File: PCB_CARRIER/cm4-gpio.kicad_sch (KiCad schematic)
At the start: 35 parts, among them J2 Micro_SD_Card_Det2, Q1 BSS138, Q3 BSS138, Q4 BC817-40, Q5 BSS138, SW1 SW_DIP_x04, U4 RT9742GGJ5

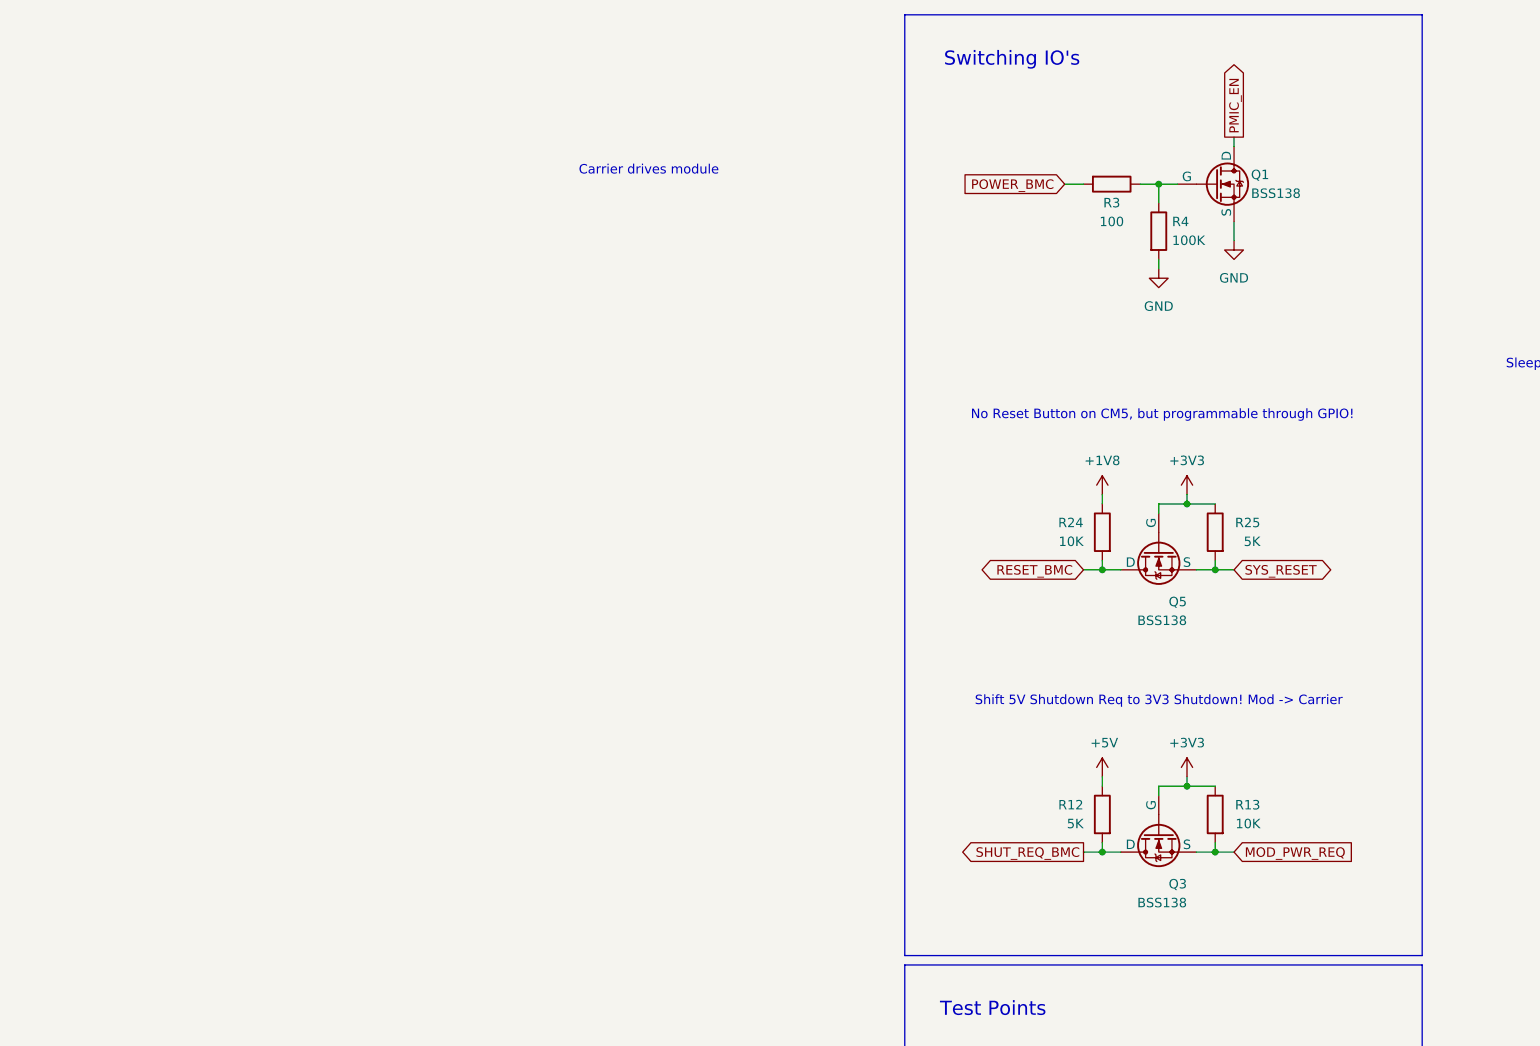
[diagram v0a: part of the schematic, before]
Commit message: fixing the PMIC mosfet
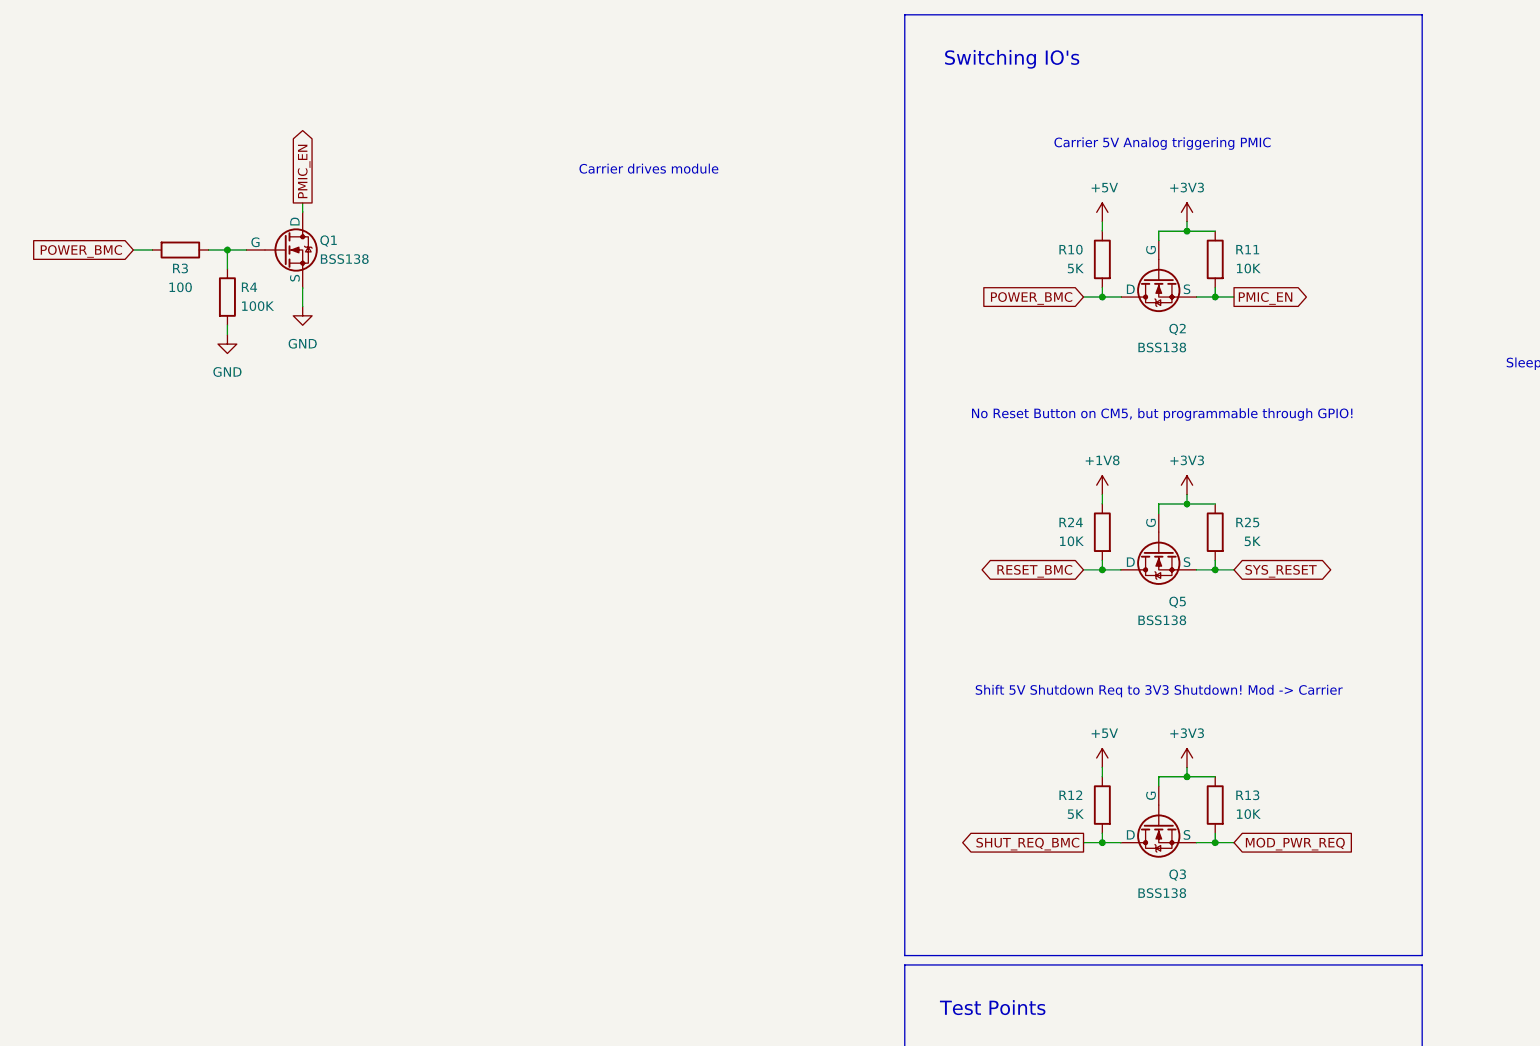
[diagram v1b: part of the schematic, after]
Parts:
- added Q2: BSS138, Package_TO_SOT_SMD:SOT-23-3, symbol Simulation_SPICE:NMOS
- added R10: 5K, Resistor_SMD:R_0402_1005Metric, symbol Device:R
- added R11: 10K, Resistor_SMD:R_0402_1005Metric, symbol Device:R
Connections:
- net +3V3: now also Q2.2 (G), R11.1
- net +5V: now also R10.1
- net PMIC_EN: now also Q2.3 (S), R11.2
- net POWER_BMC: now also Q2.1 (D), R10.2
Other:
- note added: "Carrier 5V Analog triggering PMIC"
- moved on the sheet: Q1, Q3, R12, R13, R3, R4
